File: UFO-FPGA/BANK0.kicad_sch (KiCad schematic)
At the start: 7 parts, among them U1 ICE40HX8K-BG121

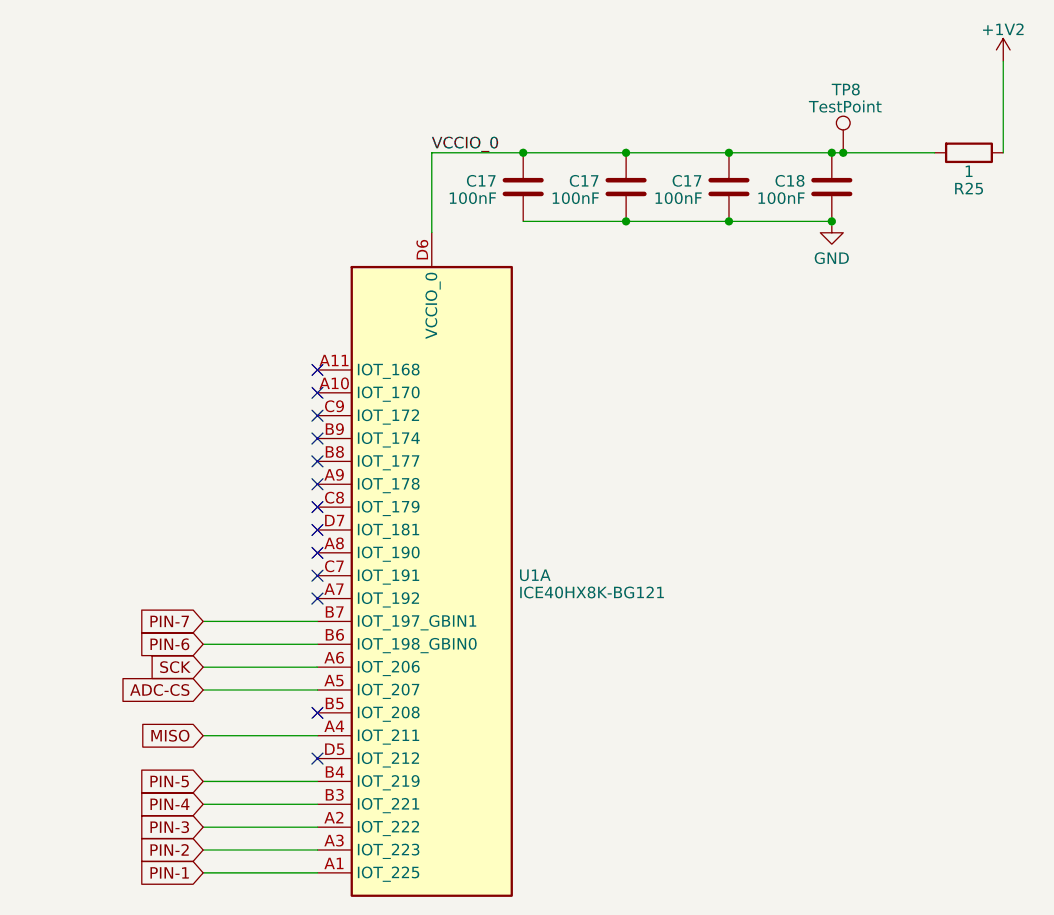
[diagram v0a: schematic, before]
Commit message: PCB
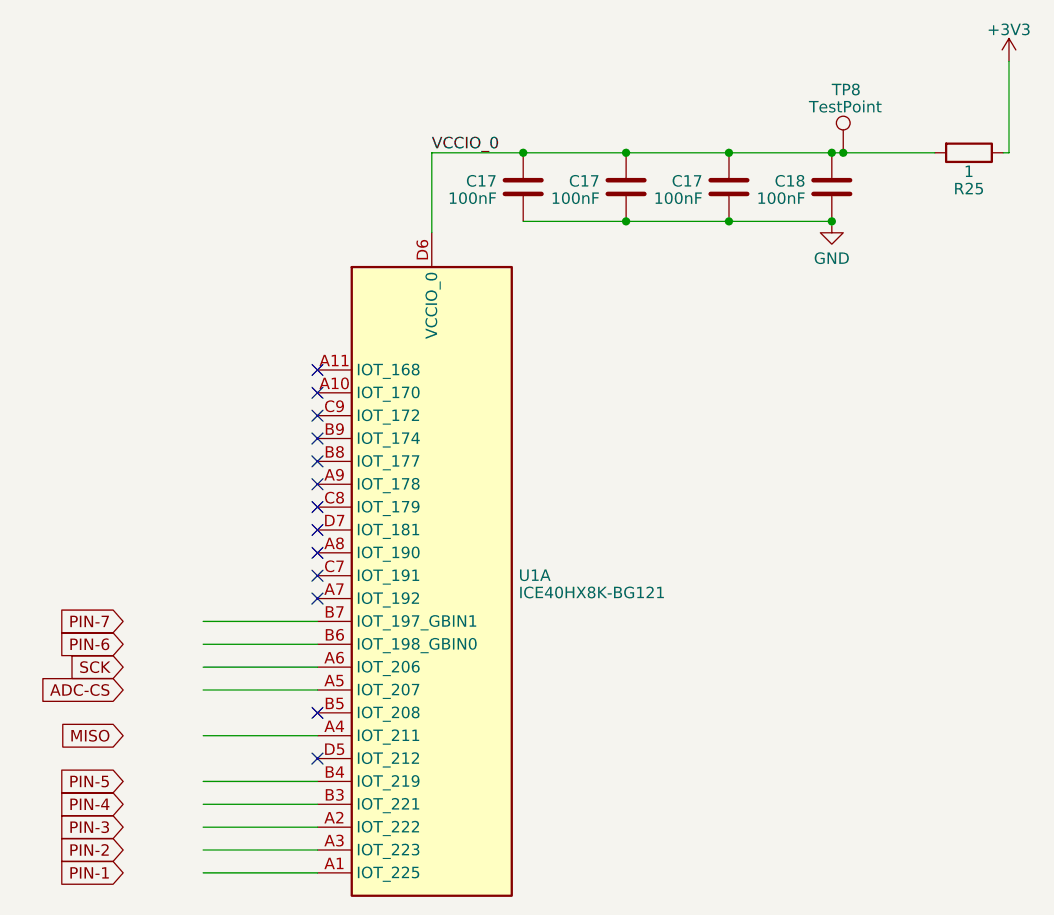
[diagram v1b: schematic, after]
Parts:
- TP8: footprint TestPoint:TestPoint_Keystone_5000-5004_Miniature -> TestPoint:TestPoint_Pad_1.5x1.5mm
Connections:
- net ADC-CS: no longer U1.A5 (IOT_207)
- net MISO: no longer U1.A4 (IOT_211)
- net PIN-1: no longer U1.A1 (IOT_225)
- net PIN-2: no longer U1.A3 (IOT_223)
- net PIN-3: no longer U1.A2 (IOT_222)
- net PIN-4: no longer U1.B3 (IOT_221)
- net PIN-5: no longer U1.B4 (IOT_219)
- net PIN-6: no longer U1.B6 (IOT_198_GBIN0)
- net PIN-7: no longer U1.B7 (IOT_197_GBIN1)
- net SCK: no longer U1.A6 (IOT_206)
- net +1V2 renamed +3V3
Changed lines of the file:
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@@
+    (stroke (width 0) (type default))
+  )
+  (wire (pts (xy 191.135 48.895) (xy 191.135 38.735))
     (stroke (width 0) (type default))
   )
@@
     (stroke (width 0) (type default))
   )
+  (wire (pts (xy 101.6 108.585) (xy 114.3 108.585))
+    (stroke (width 0) (type default))
+  )
   (wire (pts (xy 127 48.895) (xy 127 57.785))
     (stroke (width 0) (type default))
   )
-  (wire (pts (xy 101.6 108.585) (xy 114.3 108.585))
-    (stroke (width 0) (type default))
-  )
   (wire (pts (xy 160.02 56.515) (xy 148.59 56.515))
     (stroke (width 0) (type default))
@@
     (stroke (width 0) (type default))
   )
-  (wire (pts (xy 190.5 38.735) (xy 190.5 48.895))
+  (wire (pts (xy 190.5 48.895) (xy 191.135 48.895))
     (stroke (width 0) (type default))
   )
@@
     (effects (font (size 1.27 1.27)) (justify left bottom))
   )
-  (global_label "PIN-7" (shape input) (at 101.6 100.965 180) (fields_autoplaced)
-    (effects (font (size 1.27 1.27)) (justify right))
-    (property "Intersheetrefs" "${INTERSHEET_REFS}" (at 92.707 100.965 0)
-      (effects (font (size 1.27 1.27)) (justify right) hide)
-    )
-  )
-  (global_label "PIN-3" (shape input) (at 101.6 123.825 180) (fields_autoplaced)
-    (effects (font (size 1.27 1.27)) (justify right))
-    (property "Intersheetrefs" "${INTERSHEET_REFS}" (at 92.707 123.825 0)
-      (effects (font (size 1.27 1.27)) (justify right) hide)
-    )
-  )
-  (global_label "PIN-6" (shape input) (at 101.6 103.505 180) (fields_autoplaced)
-    (effects (font (size 1.27 1.27)) (justify right))
-    (property "Intersheetrefs" "${INTERSHEET_REFS}" (at 92.707 103.505 0)
-      (effects (font (size 1.27 1.27)) (justify right) hide)
-    )
-  )
-  (global_label "MISO" (shape input) (at 101.6 113.665 180) (fields_autoplaced)
-    (effects (font (size 1.27 1.27)) (justify right))
-    (property "Intersheetrefs" "${INTERSHEET_REFS}" (at 94.098 113.665 0)
-      (effects (font (size 1.27 1.27)) (justify right) hide)
-    )
-  )
-  (global_label "ADC-CS" (shape input) (at 101.6 108.585 180) (fields_autoplaced)
-    (effects (font (size 1.27 1.27)) (justify right))
-    (property "Intersheetrefs" "${INTERSHEET_REFS}" (at 91.0137 108.585 0)
-      (effects (font (size 1.27 1.27)) (justify right) hide)
-    )
-  )
-  (global_label "PIN-5" (shape input) (at 101.6 118.745 180) (fields_autoplaced)
-    (effects (font (size 1.27 1.27)) (justify right))
-    (property "Intersheetrefs" "${INTERSHEET_REFS}" (at 92.707 118.745 0)
-      (effects (font (size 1.27 1.27)) (justify right) hide)
-    )
-  )
-  (global_label "PIN-2" (shape input) (at 101.6 126.365 180) (fields_autoplaced)
-    (effects (font (size 1.27 1.27)) (justify right))
-    (property "Intersheetrefs" "${INTERSHEET_REFS}" (at 92.707 126.365 0)
-      (effects (font (size 1.27 1.27)) (justify right) hide)
-    )
-  )
-  (global_label "PIN-1" (shape input) (at 101.6 128.905 180) (fields_autoplaced)
-    (effects (font (size 1.27 1.27)) (justify right))
-    (property "Intersheetrefs" "${INTERSHEET_REFS}" (at 92.707 128.905 0)
-      (effects (font (size 1.27 1.27)) (justify right) hide)
-    )
-  )
-  (global_label "SCK" (shape input) (at 101.6 106.045 180) (fields_autoplaced)
-    (effects (font (size 1.27 1.27)) (justify right))
-    (property "Intersheetrefs" "${INTERSHEET_REFS}" (at 94.9447 106.045 0)
-      (effects (font (size 1.27 1.27)) (justify right) hide)
-    )
-  )
-  (global_label "PIN-4" (shape input) (at 101.6 121.285 180) (fields_autoplaced)
-    (effects (font (size 1.27 1.27)) (justify right))
-    (property "Intersheetrefs" "${INTERSHEET_REFS}" (at 92.707 121.285 0)
+  (global_label "PIN-7" (shape input) (at 92.71 100.965 180) (fields_autoplaced)
+    (effects (font (size 1.27 1.27)) (justify right))
+    (property "Intersheetrefs" "${INTERSHEET_REFS}" (at 83.817 100.965 0)
+      (effects (font (size 1.27 1.27)) (justify right) hide)
+    )
+  )
+  (global_label "PIN-3" (shape input) (at 92.71 123.825 180) (fields_autoplaced)
+    (effects (font (size 1.27 1.27)) (justify right))
+    (property "Intersheetrefs" "${INTERSHEET_REFS}" (at 83.817 123.825 0)
+      (effects (font (size 1.27 1.27)) (justify right) hide)
+    )
+  )
+  (global_label "PIN-6" (shape input) (at 92.71 103.505 180) (fields_autoplaced)
+    (effects (font (size 1.27 1.27)) (justify right))
+    (property "Intersheetrefs" "${INTERSHEET_REFS}" (at 83.817 103.505 0)
+      (effects (font (size 1.27 1.27)) (justify right) hide)
+    )
+  )
+  (global_label "MISO" (shape input) (at 92.71 113.665 180) (fields_autoplaced)
+    (effects (font (size 1.27 1.27)) (justify right))
+    (property "Intersheetrefs" "${INTERSHEET_REFS}" (at 85.208 113.665 0)
+      (effects (font (size 1.27 1.27)) (justify right) hide)
+    )
+  )
+  (global_label "ADC-CS" (shape input) (at 92.71 108.585 180) (fields_autoplaced)
+    (effects (font (size 1.27 1.27)) (justify right))
+    (property "Intersheetrefs" "${INTERSHEET_REFS}" (at 82.1237 108.585 0)
+      (effects (font (size 1.27 1.27)) (justify right) hide)
+    )
+  )
+  (global_label "PIN-5" (shape input) (at 92.71 118.745 180) (fields_autoplaced)
+    (effects (font (size 1.27 1.27)) (justify right))
+    (property "Intersheetrefs" "${INTERSHEET_REFS}" (at 83.817 118.745 0)
+      (effects (font (size 1.27 1.27)) (justify right) hide)
+    )
+  )
+  (global_label "PIN-2" (shape input) (at 92.71 126.365 180) (fields_autoplaced)
+    (effects (font (size 1.27 1.27)) (justify right))
+    (property "Intersheetrefs" "${INTERSHEET_REFS}" (at 83.817 126.365 0)
+      (effects (font (size 1.27 1.27)) (justify right) hide)
+    )
+  )
+  (global_label "PIN-1" (shape input) (at 92.71 128.905 180) (fields_autoplaced)
+    (effects (font (size 1.27 1.27)) (justify right))
+    (property "Intersheetrefs" "${INTERSHEET_REFS}" (at 83.817 128.905 0)
+      (effects (font (size 1.27 1.27)) (justify right) hide)
+    )
+  )
+  (global_label "SCK" (shape input) (at 92.71 106.045 180) (fields_autoplaced)
+    (effects (font (size 1.27 1.27)) (justify right))
+    (property "Intersheetrefs" "${INTERSHEET_REFS}" (at 86.0547 106.045 0)
+      (effects (font (size 1.27 1.27)) (justify right) hide)
+    )
+  )
+  (global_label "PIN-4" (shape input) (at 92.71 121.285 180) (fields_autoplaced)
+    (effects (font (size 1.27 1.27)) (justify right))
+    (property "Intersheetrefs" "${INTERSHEET_REFS}" (at 83.817 121.285 0)
       (effects (font (size 1.27 1.27)) (justify right) hide)
     )
@@
         (path "/de984c47-a4b3-4404-8f6d-5958f9d846d6"
           (reference "#PWR0101") (unit 1)
+        )
+      )
+    )
+  )
+  (symbol (lib_id "power:+3V3") (at 191.135 38.735 0) (unit 1)
+    (in_bom yes) (on_board yes) (dnp no) (fields_autoplaced)
+    (property "Reference" "#PWR062" (at 191.135 42.545 0)
+      (effects (font (size 1.27 1.27)) hide)
+    )
+    (property "Value" "+3V3" (at 191.135 35.2331 0)
+      (effects (font (size 1.27 1.27)))
+    )
+    (property "Footprint" "" (at 191.135 38.735 0)
+      (effects (font (size 1.27 1.27)) hide)
+    )
+    (property "Datasheet" "" (at 191.135 38.735 0)
+      (effects (font (size 1.27 1.27)) hide)
+    )
+    (pin "1")
+    (instances
+      (project "UFO-FPGA"
+        (path "/b3168f6a-c732-41d3-aeeb-d97dd2f1bb65/03eb349d-f783-448d-a9ad-735fd21dbf61"
+          (reference "#PWR062") (unit 1)
         )
       )
@@
     )
   )
-  (symbol (lib_id "power:+1V2") (at 190.5 38.735 0) (unit 1)
-    (in_bom yes) (on_board yes) (dnp no) (fields_autoplaced)
-    (property "Reference" "#PWR024" (at 190.5 42.545 0)
-      (effects (font (size 1.27 1.27)) hide)
-    )
-    (property "Value" "+1V2" (at 190.5 35.2331 0)
-      (effects (font (size 1.27 1.27)))
-    )
-    (property "Footprint" "" (at 190.5 38.735 0)
-      (effects (font (size 1.27 1.27)) hide)
-    )
-    (property "Datasheet" "" (at 190.5 38.735 0)
-      (effects (font (size 1.27 1.27)) hide)
-    )
-    (pin "1")
-    (instances
-      (project "UFO-FPGA"
-        (path "/b3168f6a-c732-41d3-aeeb-d97dd2f1bb65/a9a0295d-b075-4952-a5ba-04debc5f691c"
-          (reference "#PWR024") (unit 1)
-        )
-        (path "/b3168f6a-c732-41d3-aeeb-d97dd2f1bb65/03eb349d-f783-448d-a9ad-735fd21dbf61"
-          (reference "#PWR076") (unit 1)
-        )
-        (path "/b3168f6a-c732-41d3-aeeb-d97dd2f1bb65/6f7e0d88-d92b-4c4f-9dc8-64721cd46d41"
-          (reference "#PWR029") (unit 1)
-        )
-        (path "/b3168f6a-c732-41d3-aeeb-d97dd2f1bb65/f54d4357-d916-4d6b-afb9-9dd5f65d1cf7"
-          (reference "#PWR036") (unit 1)
-        )
-      )
-      (project "BANK0"
-        (path "/de984c47-a4b3-4404-8f6d-5958f9d846d6"
-          (reference "#PWR024") (unit 1)
-        )
-      )
-    )
-  )
   (symbol (lib_id "Connector:TestPoint") (at 172.72 48.895 0) (unit 1)
     (in_bom yes) (on_board yes) (dnp no)
@@
       (effects (font (size 1.27 1.27)) (justify left))
     )
-    (property "Footprint" "TestPoint:TestPoint_Keystone_5000-5004_Miniature" (at 177.8 48.895 0)
-      (effects (font (size 1.27 1.27)) hide)
-    )
+    (property "Footprint" "TestPoint:TestPoint_Pad_1.5x1.5mm" (at 177.8 48.895 0)
+      (effects (font (size 1.27 1.27)) hide)
+    )

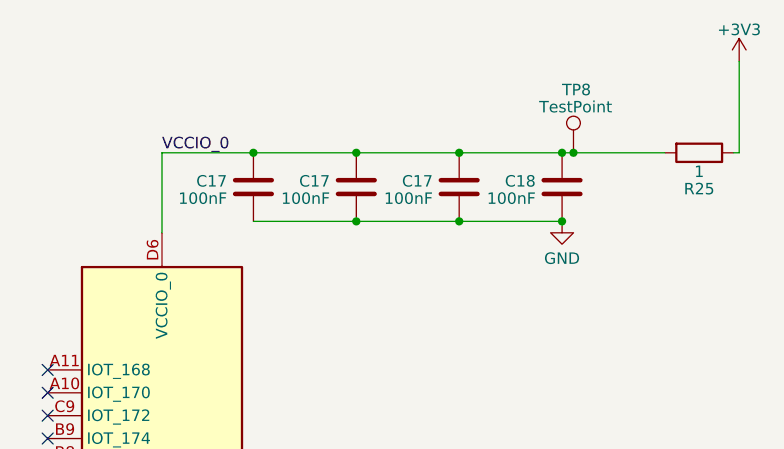
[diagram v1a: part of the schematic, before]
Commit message: PCB
many pcb changes
-started routing
-added vias
-power planes
-ground planes
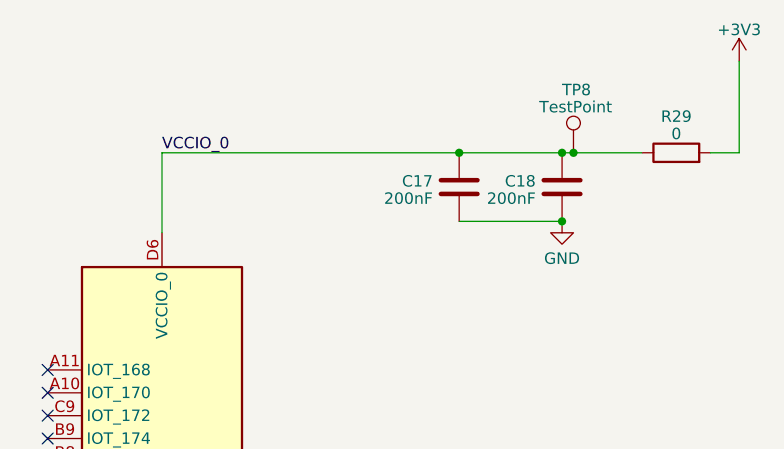
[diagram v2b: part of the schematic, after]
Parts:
- removed C17 (x2): 100nF, Capacitor_SMD:C_0805_2012Metric_Pad1.18x1.45mm_HandSolder, symbol Device:C
- removed R25: 1, Resistor_SMD:R_0805_2012Metric_Pad1.20x1.40mm_HandSolder, symbol Device:R
- added R29: 0, Resistor_SMD:R_0805_2012Metric_Pad1.20x1.40mm_HandSolder, symbol Device:R
- C17, C18: value 100nF -> 200nF
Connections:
- net +3V3: now also R29.2
- net VCCIO_0: now also R29.1
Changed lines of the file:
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@@
   (junction (at 171.45 48.895) (diameter 0) (color 0 0 0 0)
   )
-  (junction (at 160.02 56.515) (diameter 0) (color 0 0 0 0)
-  )
-  (junction (at 148.59 48.895) (diameter 0) (color 0 0 0 0)
-  )
   (junction (at 172.72 48.895) (diameter 0) (color 0 0 0 0)
-  )
-  (junction (at 137.16 48.895) (diameter 0) (color 0 0 0 0)
-  )
-  (junction (at 148.59 56.515) (diameter 0) (color 0 0 0 0)
   )
   (no_connect (at 114.3 90.805))
@@
     (stroke (width 0) (type default))
   )
+  (wire (pts (xy 187.96 48.895) (xy 191.135 48.895))
+    (stroke (width 0) (type default))
+  )
   (wire (pts (xy 101.6 100.965) (xy 114.3 100.965))
     (stroke (width 0) (type default))
@@
     (stroke (width 0) (type default))
   )
-  (wire (pts (xy 160.02 56.515) (xy 148.59 56.515))
-    (stroke (width 0) (type default))
-  )
-  (wire (pts (xy 148.59 56.515) (xy 137.16 56.515))
-    (stroke (width 0) (type default))
-  )
   (wire (pts (xy 101.6 113.665) (xy 114.3 113.665))
     (stroke (width 0) (type default))
@@
     (stroke (width 0) (type default))
   )
-  (wire (pts (xy 190.5 48.895) (xy 191.135 48.895))
+  (wire (pts (xy 172.72 48.895) (xy 180.34 48.895))
     (stroke (width 0) (type default))
   )
@@
     (stroke (width 0) (type default))
   )
-  (wire (pts (xy 148.59 48.895) (xy 137.16 48.895))
-    (stroke (width 0) (type default))
-  )
-  (wire (pts (xy 137.16 48.895) (xy 127 48.895))
-    (stroke (width 0) (type default))
-  )
-  (wire (pts (xy 160.02 48.895) (xy 148.59 48.895))
-    (stroke (width 0) (type default))
-  )
-  (wire (pts (xy 172.72 48.895) (xy 182.88 48.895))
+  (wire (pts (xy 127 48.895) (xy 160.02 48.895))
     (stroke (width 0) (type default))
   )
@@
     (property "Intersheetrefs" "${INTERSHEET_REFS}" (at 83.817 121.285 0)
       (effects (font (size 1.27 1.27)) (justify right) hide)
-    )
-  )
-  (symbol (lib_id "Device:C") (at 148.59 52.705 0) (mirror y) (unit 1)
-    (in_bom yes) (on_board yes) (dnp no) (fields_autoplaced)
-    (property "Reference" "C17" (at 145.669 52.0613 0)
-      (effects (font (size 1.27 1.27)) (justify left))
-    )
-    (property "Value" "100nF" (at 145.669 53.9823 0)
-      (effects (font (size 1.27 1.27)) (justify left))
-    )
-    (property "Footprint" "Capacitor_SMD:C_0805_2012Metric_Pad1.18x1.45mm_HandSolder" (at 147.6248 56.515 0)
-      (effects (font (size 1.27 1.27)) hide)
-    )
-    (property "Datasheet" "~" (at 148.59 52.705 0)
-      (effects (font (size 1.27 1.27)) hide)
-    )
-    (pin "1")
-    (pin "2")
-    (instances
-      (project "UFO-FPGA"
-        (path "/b3168f6a-c732-41d3-aeeb-d97dd2f1bb65/a9a0295d-b075-4952-a5ba-04debc5f691c"
-          (reference "C17") (unit 1)
-        )
-        (path "/b3168f6a-c732-41d3-aeeb-d97dd2f1bb65/6f7e0d88-d92b-4c4f-9dc8-64721cd46d41"
-          (reference "C23") (unit 1)
-        )
-        (path "/b3168f6a-c732-41d3-aeeb-d97dd2f1bb65/f54d4357-d916-4d6b-afb9-9dd5f65d1cf7"
-          (reference "C26") (unit 1)
-        )
-        (path "/b3168f6a-c732-41d3-aeeb-d97dd2f1bb65/03eb349d-f783-448d-a9ad-735fd21dbf61"
-          (reference "C30") (unit 1)
-        )
-      )
-      (project "BANK0"
-        (path "/de984c47-a4b3-4404-8f6d-5958f9d846d6"
-          (reference "C17") (unit 1)
-        )
-      )
     )
   )
@@
       (effects (font (size 1.27 1.27)) (justify left))
     )
-    (property "Value" "100nF" (at 157.099 53.9823 0)
+    (property "Value" "200nF" (at 157.099 53.9823 0)
       (effects (font (size 1.27 1.27)) (justify left))
     )
@@
     )
   )
-  (symbol (lib_id "Device:R") (at 186.69 48.895 270) (unit 1)
-    (in_bom yes) (on_board yes) (dnp no)
-    (property "Reference" "R25" (at 186.69 52.9209 90)
+  (symbol (lib_id "Device:R") (at 184.15 48.895 90) (unit 1)
+    (in_bom yes) (on_board yes) (dnp no) (fields_autoplaced)
+    (property "Reference" "R29" (at 184.15 44.8691 90)
       (effects (font (size 1.27 1.27)))
     )
-    (property "Value" "1" (at 186.69 50.9999 90)
+    (property "Value" "0" (at 184.15 46.7901 90)
       (effects (font (size 1.27 1.27)))
     )
-    (property "Footprint" "Resistor_SMD:R_0805_2012Metric_Pad1.20x1.40mm_HandSolder" (at 186.69 47.117 90)
-      (effects (font (size 1.27 1.27)) hide)
-    )
-    (property "Datasheet" "~" (at 186.69 48.895 0)
+    (property "Footprint" "Resistor_SMD:R_0805_2012Metric_Pad1.20x1.40mm_HandSolder" (at 184.15 50.673 90)
+      (effects (font (size 1.27 1.27)) hide)
+    )
+    (property "Datasheet" "~" (at 184.15 48.895 0)
       (effects (font (size 1.27 1.27)) hide)
     )
@@
     (instances
       (project "UFO-FPGA"
-        (path "/b3168f6a-c732-41d3-aeeb-d97dd2f1bb65/a9a0295d-b075-4952-a5ba-04debc5f691c"
-          (reference "R25") (unit 1)
-        )
-        (path "/b3168f6a-c732-41d3-aeeb-d97dd2f1bb65/6f7e0d88-d92b-4c4f-9dc8-64721cd46d41"
-          (reference "R28") (unit 1)
-        )
         (path "/b3168f6a-c732-41d3-aeeb-d97dd2f1bb65/f54d4357-d916-4d6b-afb9-9dd5f65d1cf7"
-          (reference "R30") (unit 1)
-        )
-        (path "/b3168f6a-c732-41d3-aeeb-d97dd2f1bb65/03eb349d-f783-448d-a9ad-735fd21dbf61"
-          (reference "R31") (unit 1)
-        )
-      )
-      (project "BANK0"
-        (path "/de984c47-a4b3-4404-8f6d-5958f9d846d6"
-          (reference "R25") (unit 1)
+          (reference "R29") (unit 1)
+        )
+        (path "/b3168f6a-c732-41d3-aeeb-d97dd2f1bb65/03eb349d-f783-448d-a9ad-735fd21dbf61"
+          (reference "R32") (unit 1)
         )
       )
@@
       (effects (font (size 1.27 1.27)) (justify left))
     )
-    (property "Value" "100nF" (at 168.529 53.9823 0)
+    (property "Value" "200nF" (at 168.529 53.9823 0)
       (effects (font (size 1.27 1.27)) (justify left))
     )
@@
         )
       )
-    )
-  )
-  (symbol (lib_id "Device:C") (at 137.16 52.705 0) (mirror y) (unit 1)
-    (in_bom yes) (on_board yes) (dnp no) (fields_autoplaced)
-    (property "Reference" "C17" (at 134.239 52.0613 0)
-      (effects (font (size 1.27 1.27)) (justify left))
-    )
-    (property "Value" "100nF" (at 134.239 53.9823 0)
-      (effects (font (size 1.27 1.27)) (justify left))
-    )
-    (property "Footprint" "Capacitor_SMD:C_0805_2012Metric_Pad1.18x1.45mm_HandSolder" (at 136.1948 56.515 0)
-      (effects (font (size 1.27 1.27)) hide)
-    )
-    (property "Datasheet" "~" (at 137.16 52.705 0)
-      (effects (font (size 1.27 1.27)) hide)
-    )
-    (pin "1")
-    (pin "2")
-    (instances
-      (project "UFO-FPGA"
-        (path "/b3168f6a-c732-41d3-aeeb-d97dd2f1bb65/a9a0295d-b075-4952-a5ba-04debc5f691c"
-          (reference "C17") (unit 1)
-        )
-        (path "/b3168f6a-c732-41d3-aeeb-d97dd2f1bb65/6f7e0d88-d92b-4c4f-9dc8-64721cd46d41"
-          (reference "C24") (unit 1)
-        )
-        (path "/b3168f6a-c732-41d3-aeeb-d97dd2f1bb65/f54d4357-d916-4d6b-afb9-9dd5f65d1cf7"
-          (reference "C25") (unit 1)
-        )
-        (path "/b3168f6a-c732-41d3-aeeb-d97dd2f1bb65/03eb349d-f783-448d-a9ad-735fd21dbf61"
-          (reference "C29") (unit 1)
-        )
-      )
-      (project "BANK0"
-        (path "/de984c47-a4b3-4404-8f6d-5958f9d846d6"
-          (reference "C17") (unit 1)
-        )
-      )
